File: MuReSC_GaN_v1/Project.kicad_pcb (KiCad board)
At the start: 4 copper layers, 71.1 x 40 mm, 112 parts, among them IC1 STM32G474RET6, IC10 UCC12040DVE, IC11 LMG1020YFFR, IC12 LMG1020YFFR, IC13 LMG1020YFFR, IC14 LMG1020YFFR, IC2 TPSM5601R5HRDAR, IC3 ISO7720FQDQ1, IC4 ISO7720FQDQ1, IC5 ISO7720FQDQ1, IC6 ISO7720FQDQ1, IC7 UCC12040DVE, IC8 UCC12040DVE, IC9 UCC12040DVE, J1 62000211121_x6, J2 62000211121, J3 62000211121_x1, J4 62000211121_x1, P1 691214110002, P2 691214110002, Q1 GS61004B-TR, Q2 GS61004B-TR, Q3 GS61004B-TR, Q4 GS61004B-TR, Y1 NX3215SA-32.768K-STD-MUS-2, Y2 NX3225SA-24.000MHZ-STD-CSR-1

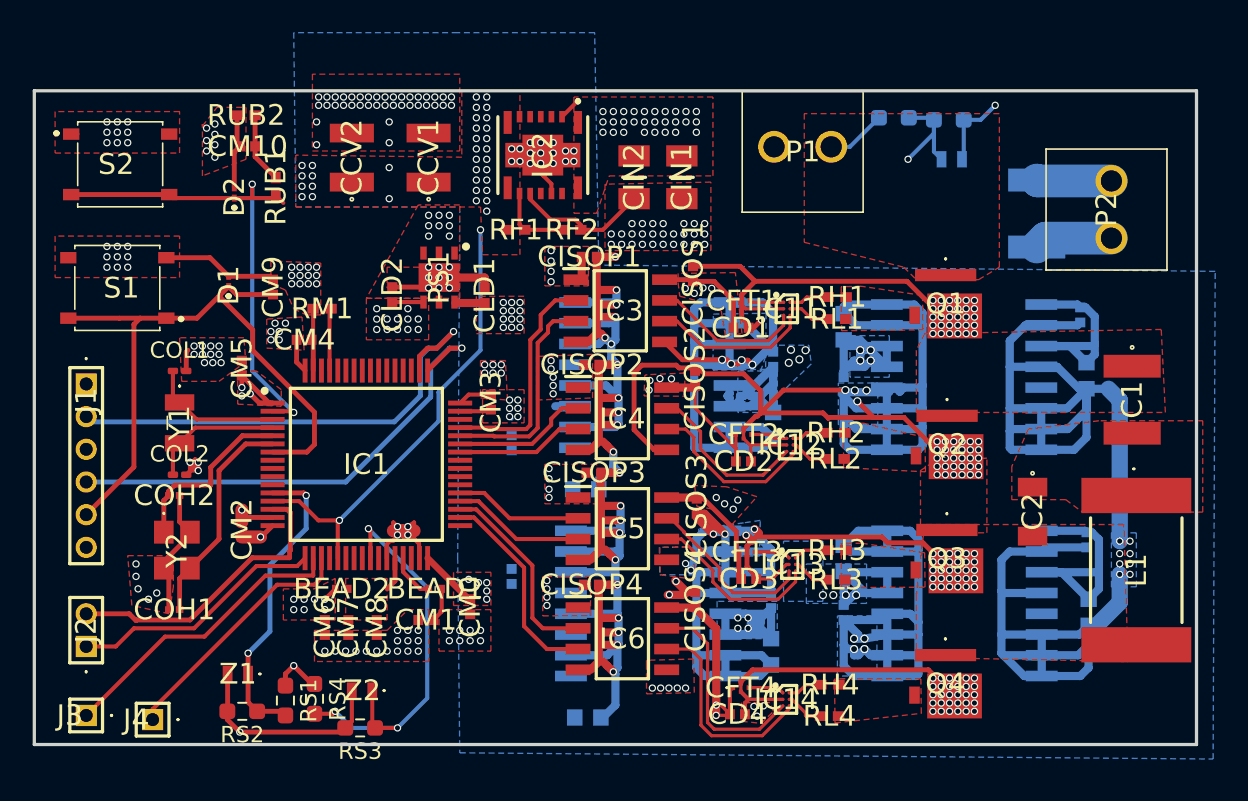
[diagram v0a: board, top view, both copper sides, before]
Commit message: LAYOUT DRC
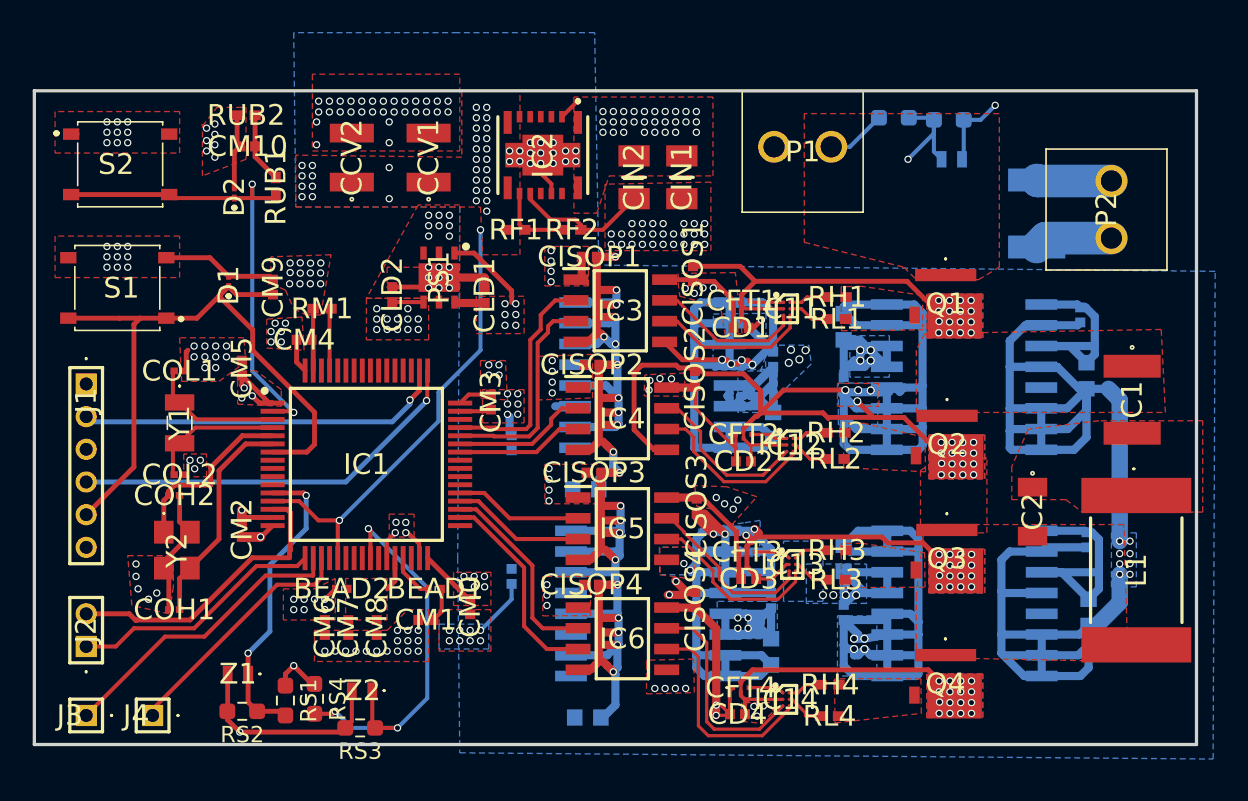
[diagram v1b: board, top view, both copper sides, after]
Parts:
- COL1, COL2: footprint Capacitor_SMD:C_0201_0603Metric_Pad0.64x0.40mm_HandSolder -> SamacSys_Parts:CAPC0603X33N
- moved J4 0.25 mm to (23.1, 117.6)
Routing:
- net /T_SWCLK: track 29.9 -> 22.7 mm
- net /T_SWDIO: track 30.1 -> 24.8 mm
- net /VDD5V: track 30.9 -> 36.1 mm, vias 45 -> 37
- net GND: track 337.8 -> 333.4 mm, vias 256 -> 232
- net /UBUTT: track 30.5 -> 29.9 mm
- net /S3: track 68.3 -> 68.5 mm, vias 36 -> 22
- net /VDD3V3: track 19.8 -> 19.7 mm, vias 66 -> 62
- net /S2: vias 35 -> 21
- net /S1: vias 35 -> 21
- added copper zone on In1.Cu, net /S1
- added copper zone on In2.Cu, net /S1
- added copper zone on In1.Cu, net /S2
- added copper zone on In1.Cu, net /S3
- added copper zone on In2.Cu, net /S3
- added copper zone on In2.Cu, net GND
